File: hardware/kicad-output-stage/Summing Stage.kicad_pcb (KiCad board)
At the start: 2 copper layers, 20 x 110 mm, 18 parts, among them IC1 TL074, J1 Thonkiconn_Mono_Jack, J2 AudioJack3

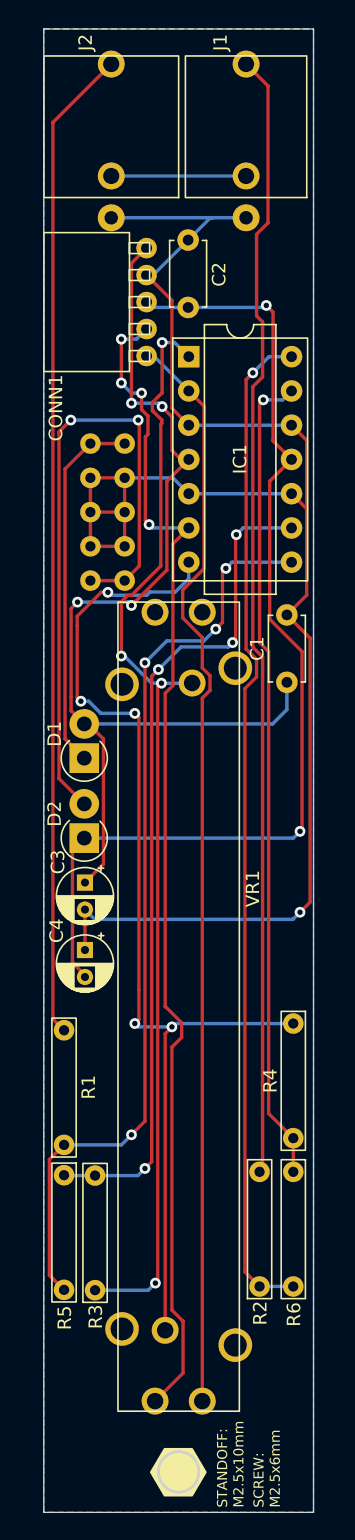
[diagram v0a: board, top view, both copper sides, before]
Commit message: Changes
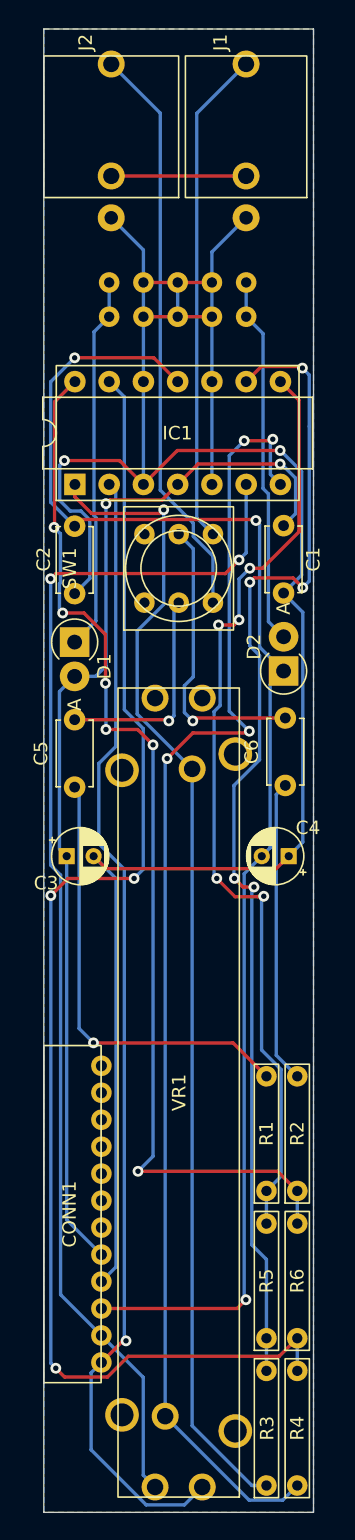
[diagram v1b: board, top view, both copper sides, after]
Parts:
- added C5: 100n, Capacitor_THT:C_Disc_D4.7mm_W2.5mm_P5.00mm, F.Cu at (2.29, 56.2)
- added C6: 100n, Capacitor_THT:C_Disc_D4.7mm_W2.5mm_P5.00mm, F.Cu at (17.9, 56.1)
- added SW1: SW_DPDT_x2, Eurorack:Sub-Miniature Toggle Switch DPDT, F.Cu at (10.0, 40.0)
- CONN1: footprint Eurorack:Header 2.0mm Right Angle Female -> Eurorack:Header 01x12 2.0mm Right Angle Female
- moved CONN1 67.6 mm to (0.00, 87.9)
- moved C2 27.5 mm to (2.29, 41.9), turned to 90 degrees
- moved R4 25.8 mm to (18.8, 103.8), turned to 90 degrees
- moved D2 19.3 mm to (17.8, 47.6)
- moved R3 19.3 mm to (16.5, 103.8)
- moved C4 16.6 mm to (18.2, 61.3), turned to 180 degrees
- moved PowerHeader1 16.6 mm to (9.93, 20.1), turned to 0 degrees
- moved R5 15.4 mm to (16.5, 92.8), turned to 90 degrees
- moved R1 15.4 mm to (16.5, 81.9)
- moved C1 11.6 mm to (17.8, 36.8), turned to -90 degrees
- moved D1 8.64 mm to (2.29, 45.5), turned to -90 degrees
- moved R2 7.62 mm to (18.8, 81.9)
- moved VR1 6.37 mm to (10.0, 78.9)
- moved IC1 5.03 mm to (9.91, 30.0), turned to 90 degrees
- moved R6 3.85 mm to (18.8, 92.8), turned to 90 degrees
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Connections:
- R1 pad 2: L OUT -> Net-(C5-Pad1)
- R2 pad 2: R OUT -> Net-(C6-Pad1)
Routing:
- net R OUT: track 84.1 -> 36.9 mm
- net Net-(IC1-Pad13): track 60.8 -> 101.9 mm, vias 1 -> 3
- net Earth: track 126.6 -> 164.2 mm, vias 1 -> 2
- net Net-(C5-Pad1): track 0.00 -> 33.4 mm, vias 0 -> 1
- net L OUT: track 73.8 -> 43.1 mm
- net -12V: track 77.7 -> 106.9 mm, vias 2 -> 3
- net Net-(IC1-Pad9): track 62.4 -> 86.9 mm, vias 4 -> 5
- net Net-(C6-Pad1): track 0.00 -> 22.5 mm
- net Net-(D2-Pad2): track 49.5 -> 27.4 mm, vias 2 -> 0
- net Net-(C6-Pad2): track 0.00 -> 21.8 mm, vias 0 -> 1
- net Net-(IC1-Pad7): track 79.5 -> 97.1 mm, vias 5 -> 4
- net Net-(C5-Pad2): track 0.00 -> 16.1 mm, vias 0 -> 1
- net Net-(IC1-Pad14): track 75.0 -> 79.9 mm, vias 1 -> 6
- net Net-(CONN1-Pad1): track 81.3 -> 84.8 mm, vias 0 -> 1
- net Net-(CONN1-Pad2): track 87.9 -> 90.9 mm, vias 4 -> 2
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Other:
- outline, holes or cut-outs redrawn
- board text added: "stackable mixer www.allensynthesis.co.uk CERN OHL-S v2 Designed in Loughborough, UK 03/04/2022"
- board text removed: "SCREW: M2.5x6mm"
- board text removed: "STANDOFF: M2.5x10mm"
- board text removed: "allen synthesis stackable mixer 05.03.2022 CERN OHL-S Designed in Loughborough UK"
